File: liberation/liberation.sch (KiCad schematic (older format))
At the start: 21 parts

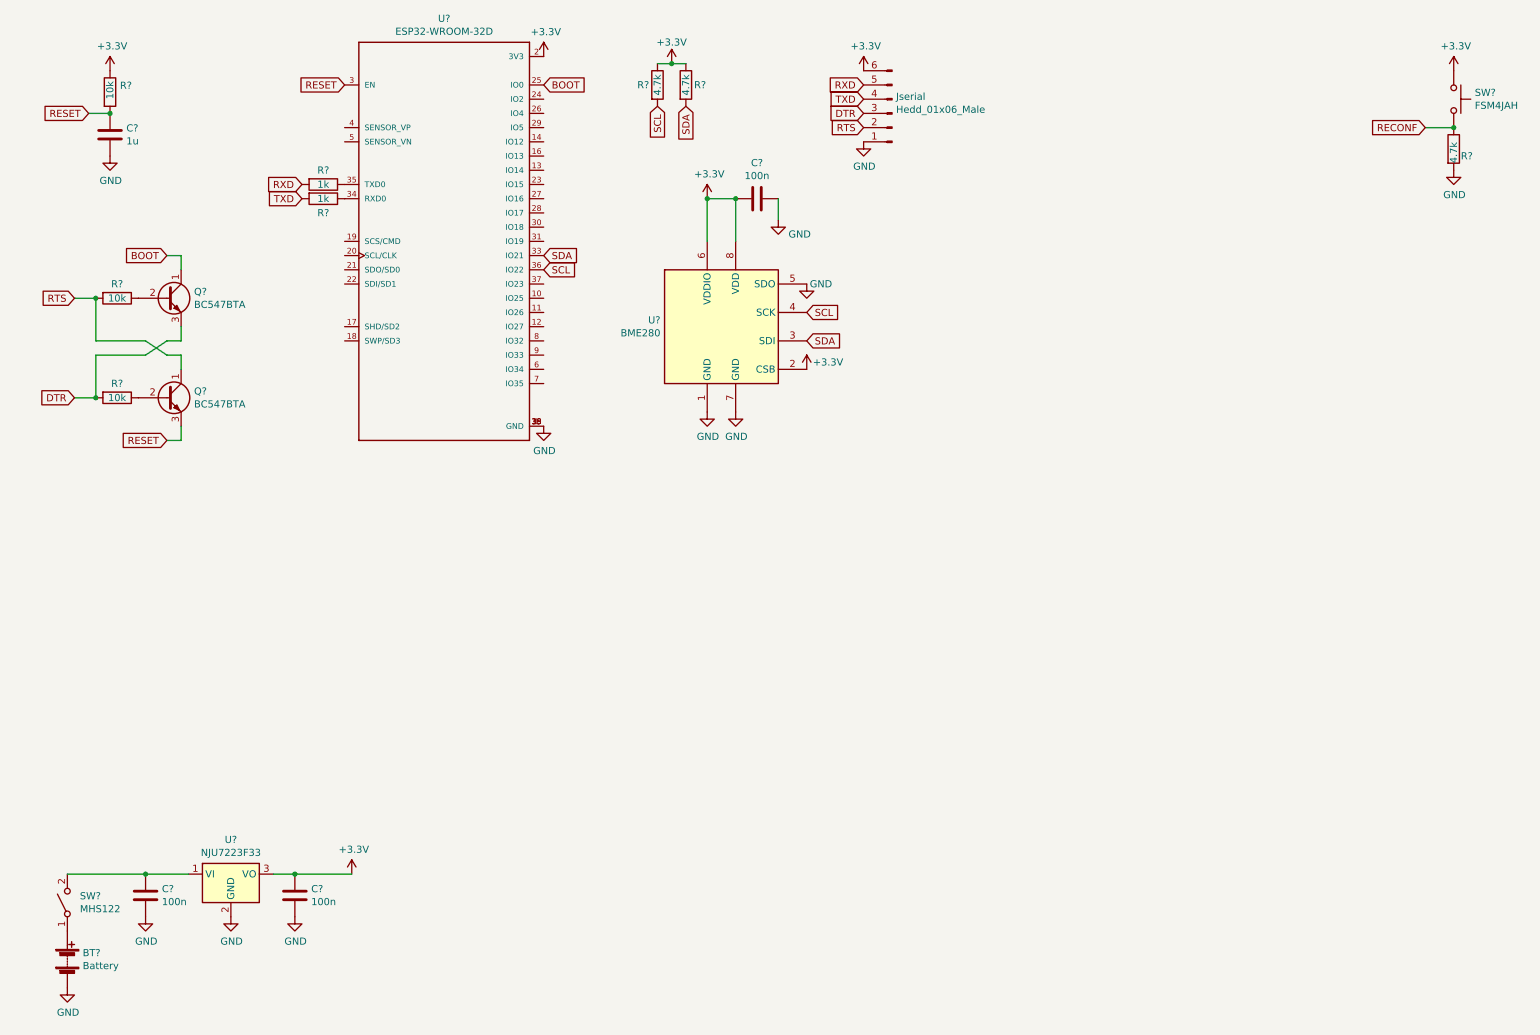
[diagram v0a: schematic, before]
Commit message: schema en netlist af
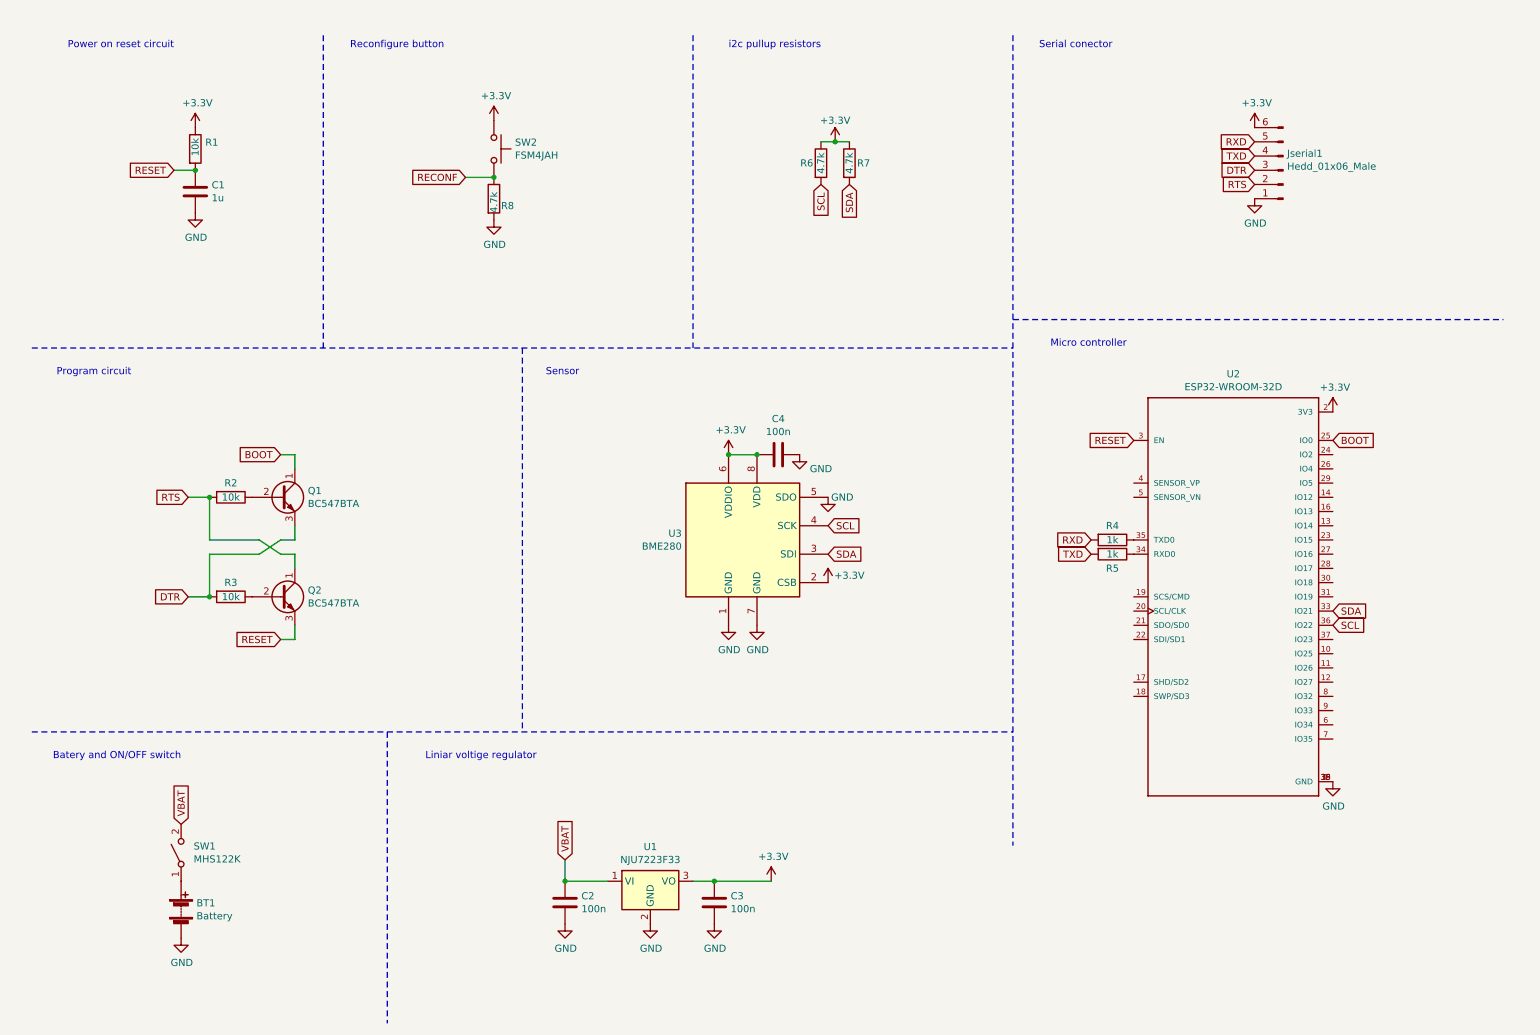
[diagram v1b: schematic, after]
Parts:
- R1, R2, R3, R4, R5, R6, R7, R8: renamed from R?; footprint (none) -> Resistor_THT:R_Axial_DIN0204_L3.6mm_D1.6mm_P7.62mm_Horizontal
- SW1: renamed from SW?; value MHS122 -> MHS122K
- SW2: renamed from SW?; footprint (none) -> Button_Switch_THT:SW_PUSH_6mm_H5mm
- U2: renamed from U?; footprint MODULE_ESP32-WROOM-32D -> ESP32-WROOM-32D:MODULE_ESP32-WROOM-32D
- gave numbers to parts that had none: 9
- renumbered Jserial to Jserial1
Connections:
- net VBAT: now reaches C2.1, SW1.2 (B), U1.1 (VI)
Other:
- note added: "Batery and ON/OFF switch"
- note added: "Liniar voltige regulator"
- note added: "Micro controller\n"
- note added: "Power on reset circuit"
- note added: "Program circuit"
- note added: "Reconfigure button\n"
- note added: "Sensor\n"
- note added: "Serial conector\n"
- note added: "i2c pullup resistors"
- moved on the sheet: BT1, C1, C2, C3, C4, Jserial1, Q1, Q2, R1, R2, R3, R4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

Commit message: scheam af nu
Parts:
- BT1: footprint (none) -> Battery:keystone_2477
- C1: footprint (none) -> Capacitor_THT:CP_Radial_D5.0mm_P2.00mm
- C2, C3, C4: footprint (none) -> Capacitor_THT:C_Disc_D4.7mm_W2.5mm_P5.00mm
- Jserial1: footprint (none) -> Connector_PinHeader_2.54mm:PinHeader_1x06_P2.54mm_Vertical
- SW1: footprint (none) -> Button_Switch_THT:MHS122
- U1: footprint (none) -> Package_TO_SOT_THT:TO-3P-3_Vertical
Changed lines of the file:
@@
 F 0 "C1" H 1915 1796 50  0000 L CNN
 F 1 "1u" H 1915 1705 50  0000 L CNN
-F 2 "" H 1838 1600 50  0001 C CNN
+F 2 "Capacitor_THT:CP_Radial_D5.0mm_P2.00mm" H 1838 1600 50  0001 C CNN
 F 3 "~" H 1800 1750 50  0001 C CNN
 	1    1800 1750
@@
 F 0 "BT1" H 1808 6846 50  0000 L CNN
 F 1 "Battery" H 1808 6755 50  0000 L CNN
-F 2 "" V 1700 6860 50  0001 C CNN
+F 2 "Battery:keystone_2477" V 1700 6860 50  0001 C CNN
 F 3 "~" V 1700 6860 50  0001 C CNN
 	1    1700 6800
@@
 F 0 "SW1" V 1746 6312 50  0000 R CNN
 F 1 "MHS122K" V 1655 6312 50  0000 R CNN
-F 2 "" H 1700 6400 50  0001 C CNN
+F 2 "Button_Switch_THT:MHS122" H 1700 6400 50  0001 C CNN
 F 3 "~" H 1700 6400 50  0001 C CNN
 	1    1700 6400
@@
 F 0 "C4" V 5648 3600 50  0000 C CNN
 F 1 "100n" V 5739 3600 50  0000 C CNN
-F 2 "" H 5938 3450 50  0001 C CNN
+F 2 "Capacitor_THT:C_Disc_D4.7mm_W2.5mm_P5.00mm" H 5938 3450 50  0001 C CNN
 F 3 "~" H 5900 3600 50  0001 C CNN
 	1    5900 3600
@@
 F 0 "U1" H 5000 6842 50  0000 C CNN
 F 1 "NJU7223F33" H 5000 6751 50  0000 C CNN
-F 2 "" H 4900 6750 50  0001 C CNN
+F 2 "Package_TO_SOT_THT:TO-3P-3_Vertical" H 4900 6750 50  0001 C CNN
 F 3 "http://ww1.microchip.com/downloads/en/devicedoc/22056b.pdf" H 5000 6850 50  0001 C CNN
 	1    5000 6600
@@
 F 0 "C2" H 4515 6796 50  0000 L CNN
 F 1 "100n" H 4515 6705 50  0000 L CNN
-F 2 "" H 4438 6600 50  0001 C CNN
+F 2 "Capacitor_THT:C_Disc_D4.7mm_W2.5mm_P5.00mm" H 4438 6600 50  0001 C CNN
 F 3 "~" H 4400 6750 50  0001 C CNN
 	1    4400 6750
@@
 F 0 "C3" H 5565 6796 50  0000 L CNN
 F 1 "100n" H 5565 6705 50  0000 L CNN
-F 2 "" H 5488 6600 50  0001 C CNN
+F 2 "Capacitor_THT:C_Disc_D4.7mm_W2.5mm_P5.00mm" H 5488 6600 50  0001 C CNN
 F 3 "~" H 5450 6750 50  0001 C CNN
 	1    5450 6750
@@
 F 0 "Jserial1" H 9422 1482 50  0000 R CNN
 F 1 "Hedd_01x06_Male" H 9422 1573 50  0000 R CNN
-F 2 "" H 9450 1600 50  0001 C CNN
+F 2 "Connector_PinHeader_2.54mm:PinHeader_1x06_P2.54mm_Vertical" H 9450 1600 50  0001 C CNN
 F 3 "~" H 9450 1600 50  0001 C CNN
 	1    9450 1600
